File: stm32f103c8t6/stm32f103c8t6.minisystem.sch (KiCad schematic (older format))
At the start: 1 part

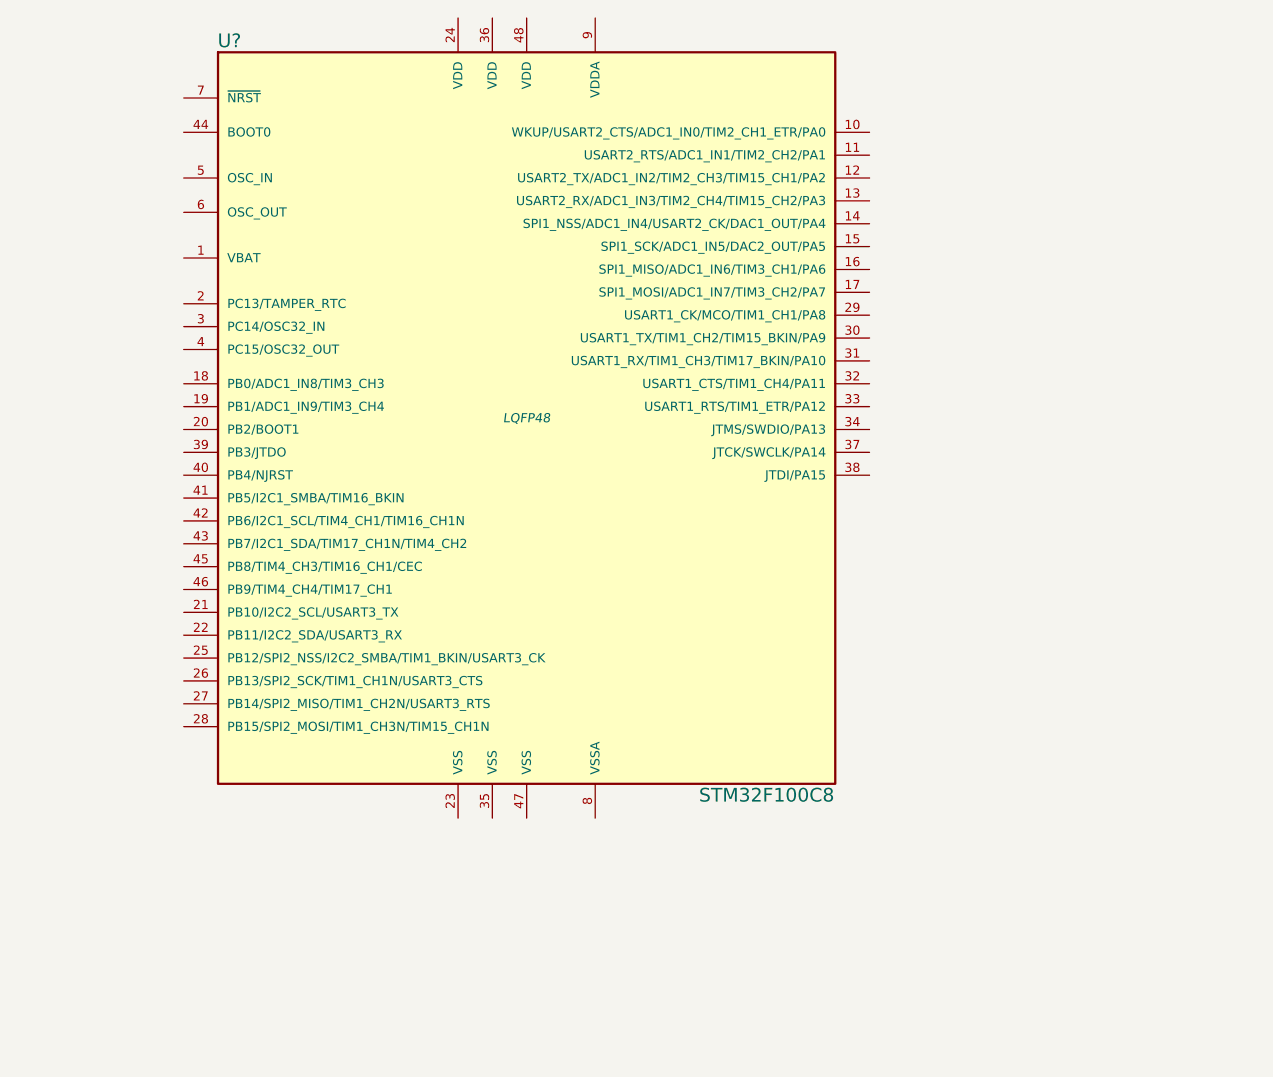
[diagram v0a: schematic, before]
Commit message: 继续原理图输入。
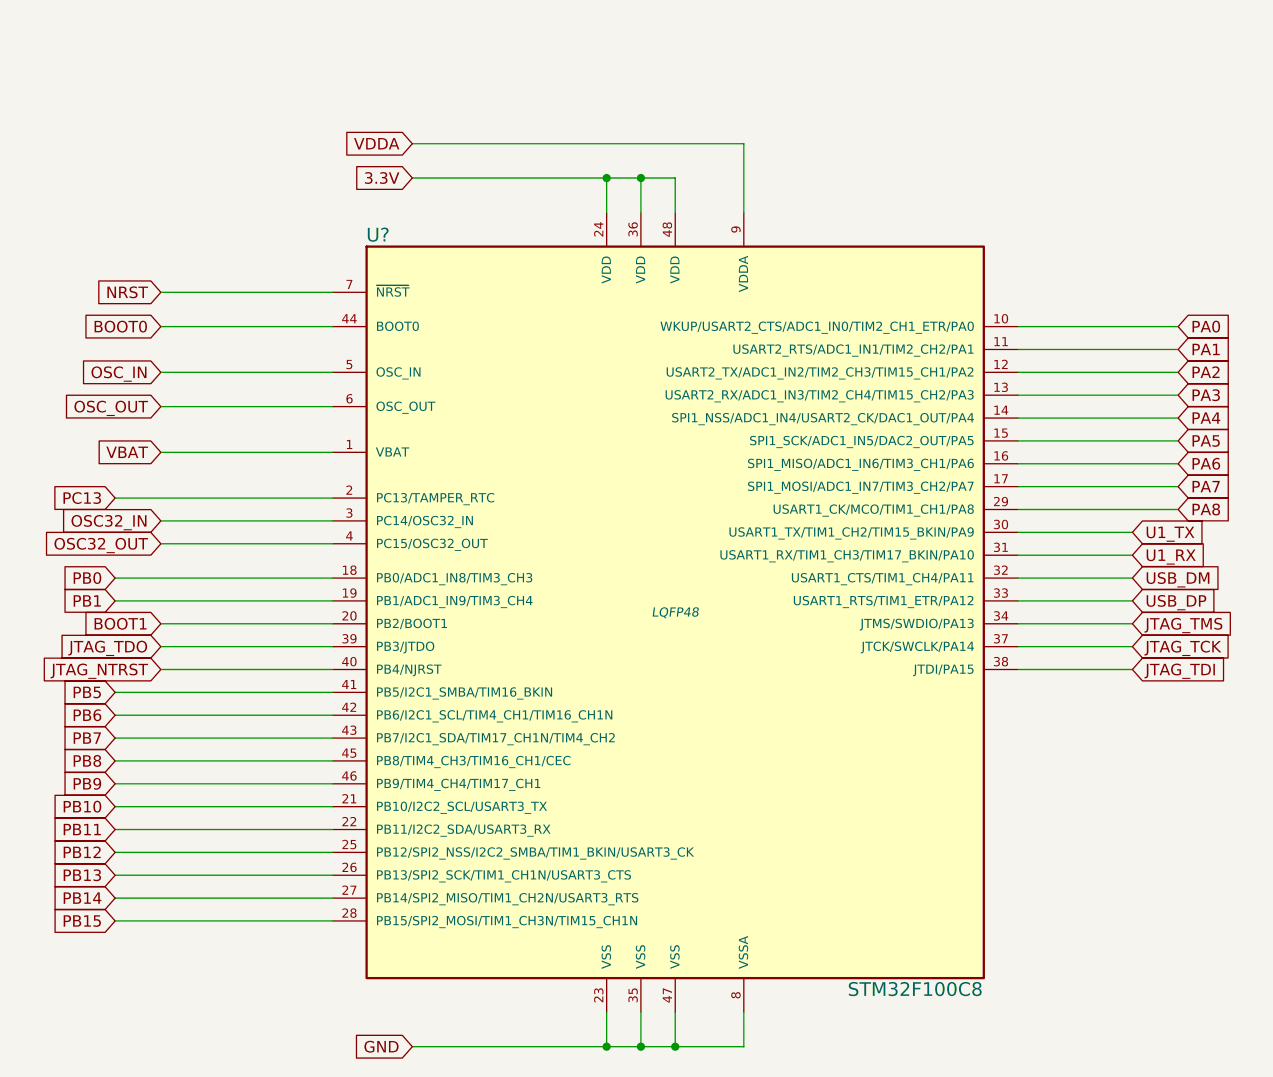
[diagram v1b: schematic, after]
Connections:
- net VBAT: now reaches U?.1 (VBAT)
- net PA0: now reaches U?.10 (WKUP/USART2_CTS/ADC1_IN0/TIM2_CH1_ETR/PA0)
- net PA1: now reaches U?.11 (USART2_RTS/ADC1_IN1/TIM2_CH2/PA1)
- net PA2: now reaches U?.12 (USART2_TX/ADC1_IN2/TIM2_CH3/TIM15_CH1/PA2)
- net PA3: now reaches U?.13 (USART2_RX/ADC1_IN3/TIM2_CH4/TIM15_CH2/PA3)
- net PA4: now reaches U?.14 (SPI1_NSS/ADC1_IN4/USART2_CK/DAC1_OUT/PA4)
- net PA5: now reaches U?.15 (SPI1_SCK/ADC1_IN5/DAC2_OUT/PA5)
- net PA6: now reaches U?.16 (SPI1_MISO/ADC1_IN6/TIM3_CH1/PA6)
- net PA7: now reaches U?.17 (SPI1_MOSI/ADC1_IN7/TIM3_CH2/PA7)
- net PB0: now reaches U?.18 (PB0/ADC1_IN8/TIM3_CH3)
- net PB1: now reaches U?.19 (PB1/ADC1_IN9/TIM3_CH4)
- net PC13: now reaches U?.2 (PC13/TAMPER_RTC)
- net BOOT1: now reaches U?.20 (PB2/BOOT1)
- net PB10: now reaches U?.21 (PB10/I2C2_SCL/USART3_TX)
- net PB11: now reaches U?.22 (PB11/I2C2_SDA/USART3_RX)
- net GND: now reaches U?.23 (VSS)
- net GND: now also U?.35 (VSS), U?.47 (VSS), U?.8 (VSSA)
- net 3.3V: now reaches U?.24 (VDD)
- net 3.3V: now also U?.36 (VDD), U?.48 (VDD)
- net PB12: now reaches U?.25 (PB12/SPI2_NSS/I2C2_SMBA/TIM1_BKIN/USART3_CK)
- net PB13: now reaches U?.26 (PB13/SPI2_SCK/TIM1_CH1N/USART3_CTS)
- net PB14: now reaches U?.27 (PB14/SPI2_MISO/TIM1_CH2N/USART3_RTS)
- net PB15: now reaches U?.28 (PB15/SPI2_MOSI/TIM1_CH3N/TIM15_CH1N)
- net PA8: now reaches U?.29 (USART1_CK/MCO/TIM1_CH1/PA8)
- net OSC32_IN: now reaches U?.3 (PC14/OSC32_IN)
- net U1_TX: now reaches U?.30 (USART1_TX/TIM1_CH2/TIM15_BKIN/PA9)
- net U1_RX: now reaches U?.31 (USART1_RX/TIM1_CH3/TIM17_BKIN/PA10)
- net USB_DM: now reaches U?.32 (USART1_CTS/TIM1_CH4/PA11)
- net USB_DP: now reaches U?.33 (USART1_RTS/TIM1_ETR/PA12)
- net JTAG_TMS: now reaches U?.34 (JTMS/SWDIO/PA13)
- net JTAG_TCK: now reaches U?.37 (JTCK/SWCLK/PA14)
- net JTAG_TDI: now reaches U?.38 (JTDI/PA15)
- net JTAG_TDO: now reaches U?.39 (PB3/JTDO)
- net OSC32_OUT: now reaches U?.4 (PC15/OSC32_OUT)
- net JTAG_NTRST: now reaches U?.40 (PB4/NJRST)
- net PB5: now reaches U?.41 (PB5/I2C1_SMBA/TIM16_BKIN)
- net PB6: now reaches U?.42 (PB6/I2C1_SCL/TIM4_CH1/TIM16_CH1N)
- net PB7: now reaches U?.43 (PB7/I2C1_SDA/TIM17_CH1N/TIM4_CH2)
- net BOOT0: now reaches U?.44 (BOOT0)
- net PB8: now reaches U?.45 (PB8/TIM4_CH3/TIM16_CH1/CEC)
- net PB9: now reaches U?.46 (PB9/TIM4_CH4/TIM17_CH1)
- net OSC_IN: now reaches U?.5 (OSC_IN)
- net OSC_OUT: now reaches U?.6 (OSC_OUT)
- net NRST: now reaches U?.7 (~NRST)
- net VDDA: now reaches U?.9 (VDDA)
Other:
- moved on the sheet: U?
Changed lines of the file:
@@
 L STM32F100C8 U?
 U 1 1 55CDB53A
-P 2750 2850
-F 0 "U?" H 1450 4500 60  0000 C CNN
-F 1 "STM32F100C8" H 3800 1200 60  0000 C CNN
-F 2 "LQFP48" H 2750 2850 40  0000 C CIN
-F 3 "" H 2750 2850 60  0000 C CNN
-	1    2750 2850
+P 3400 3700
+F 0 "U?" H 2100 5350 60  0000 C CNN
+F 1 "STM32F100C8" H 4450 2050 60  0000 C CNN
+F 2 "LQFP48" H 3400 3700 40  0000 C CIN
+F 3 "" H 3400 3700 60  0000 C CNN
+	1    3400 3700
 	1    0    0    -1
 $EndComp
+Text GLabel 1150 3300 0    50   Input ~ 0
+OSC32_IN
+Text GLabel 1150 3400 0    50   Input ~ 0
+OSC32_OUT
+Wire Wire Line
+	1150 3300 1900 3300
+Wire Wire Line
+	1900 3400 1150 3400
+Text GLabel 1150 2650 0    50   Input ~ 0
+OSC_IN
+Text GLabel 1150 2800 0    50   Input ~ 0
+OSC_OUT
+Wire Wire Line
+	1900 2650 1150 2650
+Wire Wire Line
+	1900 2800 1150 2800
+Text GLabel 1150 2300 0    50   Input ~ 0
+NRST
+Text GLabel 1150 2450 0    50   Input ~ 0
+BOOT0
+Text GLabel 1150 3750 0    50   Input ~ 0
+BOOT1
+Text GLabel 1150 3950 0    50   Input ~ 0
+JTAG_NTRST
+Text GLabel 1150 3000 0    50   Input ~ 0
+VBAT
+Text GLabel 950  3550 0    50   Input ~ 0
+PB0
+Text GLabel 950  3650 0    50   Input ~ 0
+PB1
+Text GLabel 1150 3850 0    50   Input ~ 0
+JTAG_TDO
+Text GLabel 950  4050 0    50   Input ~ 0
+PB5
+Text GLabel 950  4150 0    50   Input ~ 0
+PB6
+Text GLabel 950  4250 0    50   Input ~ 0
+PB7
+Text GLabel 950  4350 0    50   Input ~ 0
+PB8
+Text GLabel 950  4450 0    50   Input ~ 0
+PB9
+Text GLabel 950  4550 0    50   Input ~ 0
+PB10
+Text GLabel 950  4650 0    50   Input ~ 0
+PB11
+Text GLabel 950  4750 0    50   Input ~ 0
+PB12
+Text GLabel 950  4850 0    50   Input ~ 0
+PB13
+Text GLabel 950  4950 0    50   Input ~ 0
+PB14
+Text GLabel 950  5050 0    50   Input ~ 0
+PB15
+Wire Wire Line
+	1900 3000 1150 3000
+Wire Wire Line
+	1900 3550 950  3550
+Wire Wire Line
+	1900 3650 950  3650
+Wire Wire Line
+	1900 3750 1150 3750
+Wire Wire Line
+	1900 3850 1150 3850
+Wire Wire Line
+	1900 3950 1150 3950
+Wire Wire Line
+	1900 4050 950  4050
+Wire Wire Line
+	1900 4150 950  4150
+Wire Wire Line
+	1900 4250 950  4250
+Wire Wire Line
+	1900 4350 950  4350
+Wire Wire Line
+	1900 4450 950  4450
+Wire Wire Line
+	1900 4550 950  4550
+Wire Wire Line
+	1900 4650 950  4650
+Wire Wire Line
+	1900 4750 950  4750
+Wire Wire Line
+	1900 4850 950  4850
+Wire Wire Line
+	1900 4950 950  4950
+Wire Wire Line
+	1900 5050 950  5050
+Wire Wire Line
+	1900 2450 1150 2450
+Wire Wire Line
+	1900 2300 1150 2300
+Text GLabel 950  3200 0    50   Input ~ 0
+PC13
+Wire Wire Line
+	1900 3200 950  3200
+Text GLabel 2250 1800 0    50   Input ~ 0
+3.3V
+Text GLabel 2250 5600 0    50   Input ~ 0
+GND
+Wire Wire Line
+	3100 5450 3100 5600
+Wire Wire Line
+	3700 5450 3700 5600
+Wire Wire Line
+	3400 5450 3400 5600
+Wire Wire Line
+	3250 5450 3250 5600
+Wire Wire Line
+	3700 5600 2250 5600
+Connection ~ 3400 5600
+Connection ~ 3250 5600
+Connection ~ 3100 5600
+Wire Wire Line
+	3400 1950 3400 1800
+Wire Wire Line
+	3250 1950 3250 1800
+Wire Wire Line
+	3100 1950 3100 1800
+Wire Wire Line
+	3400 1800 2250 1800
+Connection ~ 3250 1800
+Connection ~ 3100 1800
+Text GLabel 2250 1650 0    50   Input ~ 0
+VDDA
+Wire Wire Line
+	3700 1950 3700 1650
+Wire Wire Line
+	3700 1650 2250 1650
+Wire Wire Line
+	4900 3350 5400 3350
+Wire Wire Line
+	4900 3450 5400 3450
+Text GLabel 5400 3350 2    50   Input ~ 0
+U1_TX
+Text GLabel 5400 3450 2    50   Input ~ 0
+U1_RX
+Text GLabel 5400 3550 2    50   Input ~ 0
+USB_DM
+Text GLabel 5400 3650 2    50   Input ~ 0
+USB_DP
+Text GLabel 5400 3750 2    50   Input ~ 0
+JTAG_TMS
+Text GLabel 5400 3850 2    50   Input ~ 0
+JTAG_TCK
+Text GLabel 5400 3950 2    50   Input ~ 0
+JTAG_TDI
+Text GLabel 5600 2450 2    50   Input ~ 0
+PA0
+Text GLabel 5600 2550 2    50   Input ~ 0
+PA1
+Text GLabel 5600 2650 2    50   Input ~ 0
+PA2
+Text GLabel 5600 2750 2    50   Input ~ 0
+PA3
+Text GLabel 5600 2850 2    50   Input ~ 0
+PA4
+Text GLabel 5600 2950 2    50   Input ~ 0
+PA5
+Text GLabel 5600 3050 2    50   Input ~ 0
+PA6
+Text GLabel 5600 3150 2    50   Input ~ 0
+PA7
+Text GLabel 5600 3250 2    50   Input ~ 0
+PA8
+Wire Wire Line
+	4900 2450 5600 2450
+Wire Wire Line
+	4900 2550 5600 2550
+Wire Wire Line
+	4900 2650 5600 2650
+Wire Wire Line
+	4900 2750 5600 2750
+Wire Wire Line
+	4900 2850 5600 2850
+Wire Wire Line
+	4900 2950 5600 2950
+Wire Wire Line
+	4900 3050 5600 3050
+Wire Wire Line
+	4900 3150 5600 3150
+Wire Wire Line
+	4900 3250 5600 3250
+Wire Wire Line
+	4900 3550 5400 3550
+Wire Wire Line
+	4900 3650 5400 3650
+Wire Wire Line
+	4900 3750 5400 3750
+Wire Wire Line
+	4900 3850 5400 3850
+Wire Wire Line
+	4900 3950 5400 3950
 $EndSCHEMATC
